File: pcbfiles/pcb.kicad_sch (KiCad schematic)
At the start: 236 parts, among them J1 Conn_01x06, J2 Conn_01x06, J3 Conn_01x06, J4 Conn_01x06, J5 Conn_01x04_Female, J6 Conn_01x04_Female, Q1 AO3401A, Q2 AO3401A, SW1 SW_SPST, SW10 SW_SPST, SW11 SW_SPST, SW12 SW_SPST, SW13 SW_SPST, SW14 SW_SPST, SW15 SW_SPST, SW16 SW_SPST, SW17 SW_SPST, SW18 SW_SPST, SW19 SW_SPST, SW2 SW_SPST, SW20 SW_SPST, SW21 SW_SPST, SW22 SW_SPST, SW23 SW_SPST, SW24 SW_SPST, SW25 SW_SPST, SW26 SW_SPST, SW27 SW_SPST, SW28 SW_SPST, SW29 SW_SPST, SW3 SW_SPST, SW30 SW_SPST, SW31 SW_SPST, SW32 SW_SPST, SW33 SW_SPST, SW34 SW_SPST, SW35 SW_SPST, SW36 SW_SPST, SW37 SW_SPST, SW38 SW_SPST, SW39 SW_SPST, SW4 SW_SPST, SW40 SW_SPST, SW41 SW_SPST, SW42 SW_SPST, SW43 SW_SPST, SW44 SW_SPST, SW45 SW_SPST, SW46 SW_SPST, SW47 SW_SPST, SW48 SW_SPST, SW49 SW_SPST, SW5 SW_SPST, SW50 SW_SPST, SW51 SW_SPST, SW52 SW_SPST, SW53 SW_SPST, SW54 SW_SPST, SW55 SW_SPST, SW56 SW_SPST, SW57 SW_SPST, SW58 SW_SPST, SW59 SW_SPST, SW6 SW_SPST, SW60 SW_SPST, SW61 SW_SPST, SW62 SW_SPST, SW63 SW_SPST, SW64 SW_SPST, SW65 SW_SPST, SW66 SW_SPST, SW67 SW_SPST, SW68 SW_SPST, SW69 SW_SPST, SW7 SW_SPST, SW70 SW_SPST, SW71 SW_SPST, SW72 SW_SPST, SW73 SW_SPST, SW74 SW_SPST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

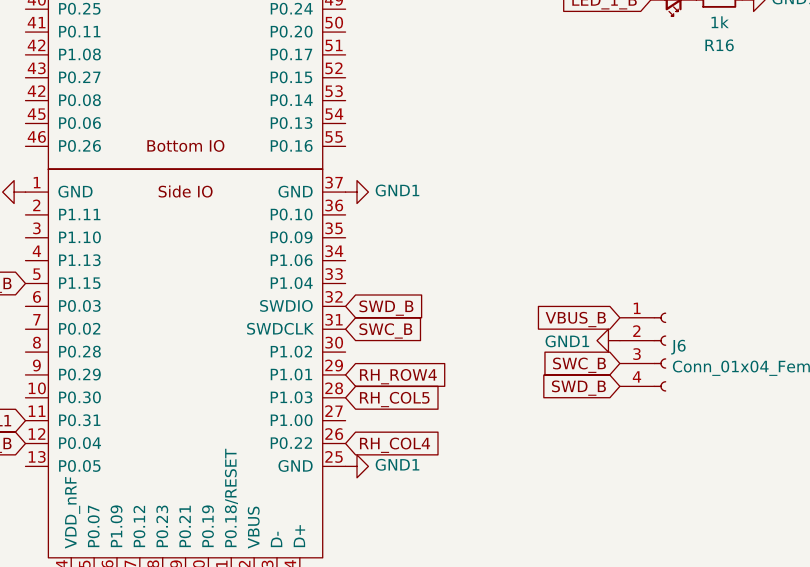
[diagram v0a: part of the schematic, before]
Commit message: Routing
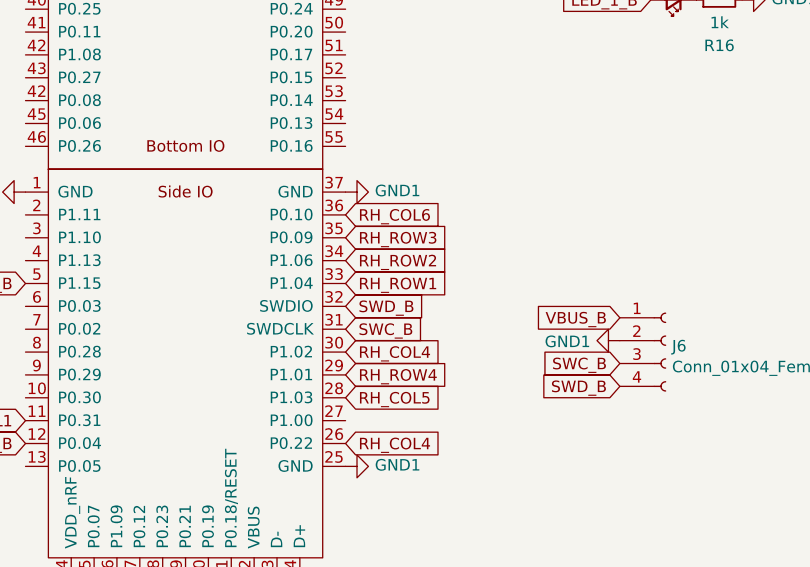
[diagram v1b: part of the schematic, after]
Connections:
- net RH_COL4: now also U6.30 (P1.02)
- net RH_COL6: now also U6.36 (P0.10)
- net RH_ROW1: now also U6.33 (P1.04)
- net RH_ROW2: now also U6.34 (P1.06)
- net RH_ROW3: now also U6.35 (P0.09)
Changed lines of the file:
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@@
+    )
+  )
+  (global_label "RH_ROW2" (shape input) (at 525.272 252.73 0) (fields_autoplaced)
+    (effects (font (size 1.27 1.27)) (justify left))
+    (property "Intersheet References" "${INTERSHEET_REFS}" (id 0) (at -130.048 133.35 0)
+      (effects (font (size 1.27 1.27)) hide)
     )
   )
@@
     )
   )
+  (global_label "RH_ROW1" (shape input) (at 525.272 255.27 0) (fields_autoplaced)
+    (effects (font (size 1.27 1.27)) (justify left))
+    (property "Intersheet References" "${INTERSHEET_REFS}" (id 0) (at 536.4257 255.1906 0)
+      (effects (font (size 1.27 1.27)) (justify left) hide)
+    )
+  )
   (global_label "RAW_B" (shape input) (at 568.96 151.892 180) (fields_autoplaced)
     (effects (font (size 1.27 1.27)) (justify right))
@@
     )
   )
+  (global_label "RH_ROW3" (shape input) (at 525.272 250.19 0) (fields_autoplaced)
+    (effects (font (size 1.27 1.27)) (justify left))
+    (property "Intersheet References" "${INTERSHEET_REFS}" (id 0) (at -130.048 120.65 0)
+      (effects (font (size 1.27 1.27)) hide)
+    )
+  )
   (global_label "VBUS_B" (shape input) (at 574.548 163.322 90) (fields_autoplaced)
     (effects (font (size 1.27 1.27)) (justify left))
@@
     )
   )
+  (global_label "RH_COL4" (shape input) (at 525.272 262.89 0) (fields_autoplaced)
+    (effects (font (size 1.27 1.27)) (justify left))
+    (property "Intersheet References" "${INTERSHEET_REFS}" (id 0) (at 609.092 -346.71 0)
+      (effects (font (size 1.27 1.27)) hide)
+    )
+  )
   (global_label "VBAT" (shape input) (at 132.842 168.91 0) (fields_autoplaced)
     (effects (font (size 1.27 1.27)) (justify left))
@@
     )
   )
+  (global_label "RH_COL6" (shape input) (at 525.272 247.65 0) (fields_autoplaced)
+    (effects (font (size 1.27 1.27)) (justify left))
+    (property "Intersheet References" "${INTERSHEET_REFS}" (id 0) (at 609.092 -397.51 0)
+      (effects (font (size 1.27 1.27)) hide)
+    )
+  )
